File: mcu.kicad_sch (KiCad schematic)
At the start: 65 parts, among them J10 PinHeader_2x10_P1.27mm_SMD_Sh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, SW5 SW_B3U-1000P_SMD, SW6 CAS-120TA, U1 STM32H753ZIT6, Y1 Resonator_32.768kHz_ECX-31B, Y2 Oscillator_25MHz_ESC_2016MV

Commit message: [#95036] Rearrange MCU scheet
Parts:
- removed R172: R_10k_0402, antmicro-footprints:R_0402_1005Metric, symbol antmicroResistors0402:R_10k_0402
- added D22: RB521S30T1G, antmicro-footprints:SOD-523, symbol antmicroDiodesRectifiersSingle:RB521S30T1G
- added R175: R_2k2_0402, antmicro-footprints:R_0402_1005Metric, symbol antmicroResistors0402:R_2k2_0402
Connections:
- net JTAG.RST is gone; now on net JTAG.~{RST}: J10.10
- net +3V3: now also D22.2 (A)
- net GND: now also BT1.2 (-), J10.11, J10.13, J10.9
- net MCU_VBAT: now also D22.1 (C), R175.2
- net MCU_VDDA: now also J10.1
- net at BT1.1 (+): now also R175.1
- net SPI_2.MISO renamed SPI_2.MISO_IO1
- net SPI_2.MOSI renamed SPI_2.MOSI_IO0
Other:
- note added: "STM32H753 MCU"
- note removed: "TODO: Verify all UARTs RX/TX cross. Should I make one?"
- moved on the sheet: BT1, C14, C15, C16, C17, C18, C19, C20, C21, C22, C23, C24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

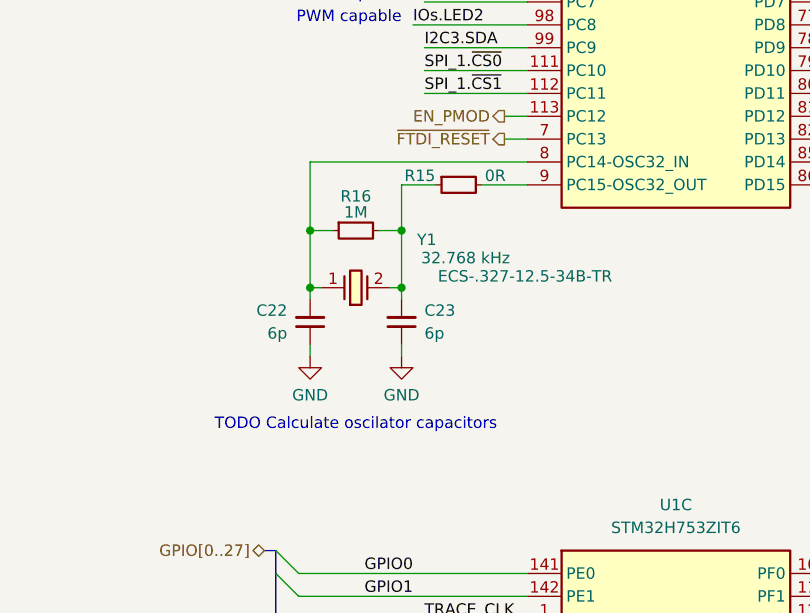
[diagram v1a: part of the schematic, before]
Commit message: [#95036] Adjust MCU LSE clock
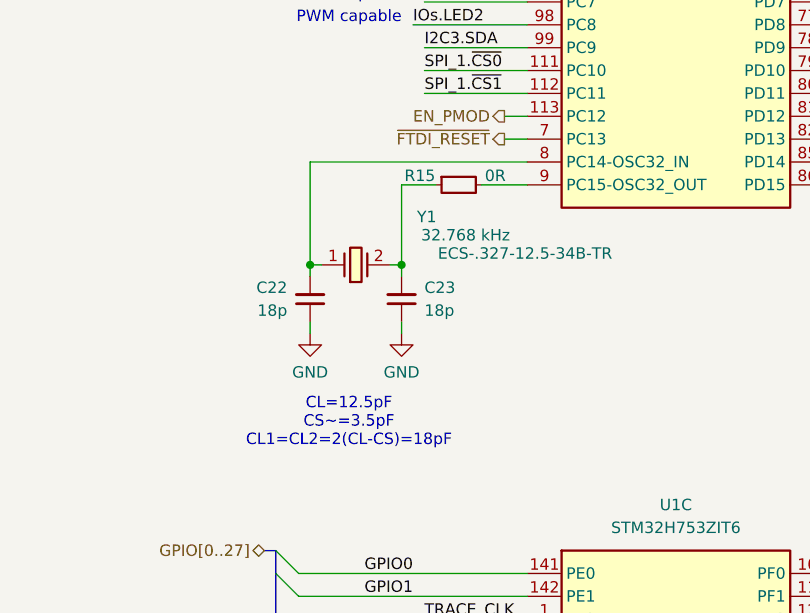
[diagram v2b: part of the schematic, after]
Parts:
- removed C22, C23: C_6p_0402, antmicro-footprints:C_0402_1005Metric, symbol antmicroCapacitors0402:C_6p_0402
- removed R16: R_1M_0402, antmicro-footprints:R_0402_1005Metric, symbol antmicroResistors0402:R_1M_0402
- added C22, C23: C_18p_0402, antmicro-footprints:C_0402_1005Metric, symbol antmicroCapacitors0402:C_18p_0402
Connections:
- net GND: now also C22.1, C23.1
- net at U1.8 (PC14-OSC32_IN), Y1.1: now also C22.2
- net at R15.1, Y1.2: now also C23.2
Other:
- note added: "CL=12.5pF CS~=3.5pF CL1=CL2=2(CL-CS)=18pF"
- note removed: "TODO Calculate oscilator capacitors"
- moved on the sheet: Y1
